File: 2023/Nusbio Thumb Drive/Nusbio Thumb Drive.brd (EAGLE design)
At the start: 26.5 x 23.5 mm, 4 parts

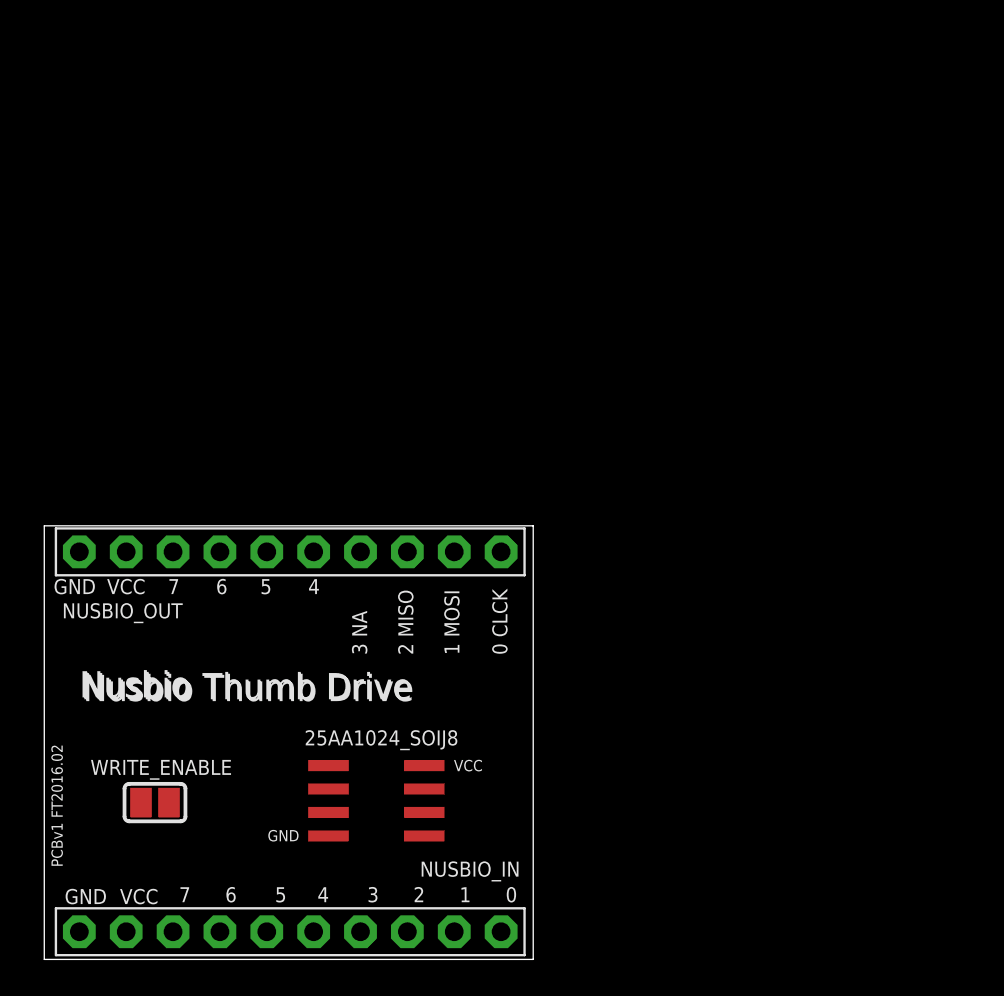
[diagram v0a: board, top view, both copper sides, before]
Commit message: new ft232 board 2023
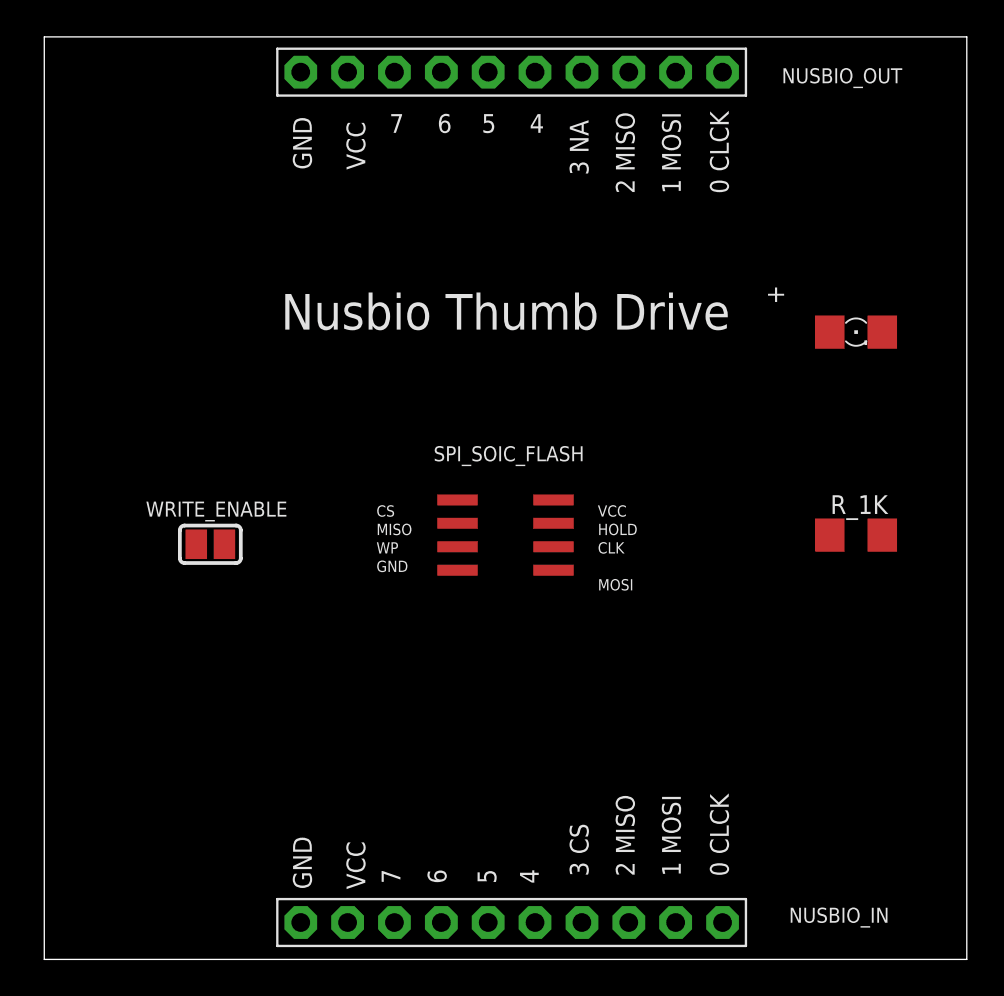
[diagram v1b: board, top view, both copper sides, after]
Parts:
- removed 25AA1024_SOIJ8: 25AA080SN, microchip:SO-08
- added LED_POWER: (no value), adafruit:1206
- added R_1K: (no value), adafruit:R1206
- added SPI_SOIC_FLASH: 25AA080SN, microchip:SO-08
- moved NUSBIO_OUT 28.6 mm to (25.3, 48.1)
- moved WRITE_ENABLE 14.3 mm to (9.00, 22.5)
- moved NUSBIO_IN 12.0 mm to (25.3, 2.00)
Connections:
- new net N$2: LED_POWER.C, R_1K.2
- net CS: now also SPI_SOIC_FLASH.1; no longer 25AA1024_SOIJ8.1
- net GND: now also R_1K.1, SPI_SOIC_FLASH.4; no longer 25AA1024_SOIJ8.4
- net MISO: now also SPI_SOIC_FLASH.2; no longer 25AA1024_SOIJ8.2
- net MOSI: now also SPI_SOIC_FLASH.5; no longer 25AA1024_SOIJ8.5
- net N$1: now also SPI_SOIC_FLASH.3; no longer 25AA1024_SOIJ8.3
- net SCK: now also SPI_SOIC_FLASH.6; no longer 25AA1024_SOIJ8.6
- net VCC: now also LED_POWER.A, SPI_SOIC_FLASH.7, SPI_SOIC_FLASH.8; no longer 25AA1024_SOIJ8.7, 25AA1024_SOIJ8.8
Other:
- board size 26.5 x 23.5 mm -> 50 x 50 mm
- board text added: "+"
- board text added: "3 CS"
- board text added: "CLK"
- board text added: "CS"
- board text added: "HOLD"
- board text added: "MISO"
- board text added: "MOSI"
- board text added: "WP"
- board text removed: "0"
- board text removed: "1"
- board text removed: "2"
- board text removed: "3"
- board text removed: "Nusbio"
- board text removed: "PCBv1 FT2016.02"
